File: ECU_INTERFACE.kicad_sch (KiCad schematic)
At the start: 14 parts, among them J10 5569-16A2, J2 5569-20A2, J3 5569-06A2, J4 5569-08A2, J5 5569-18A2

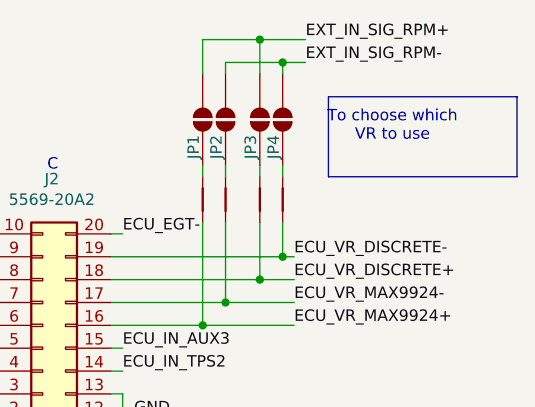
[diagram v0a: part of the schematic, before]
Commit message: Autosave
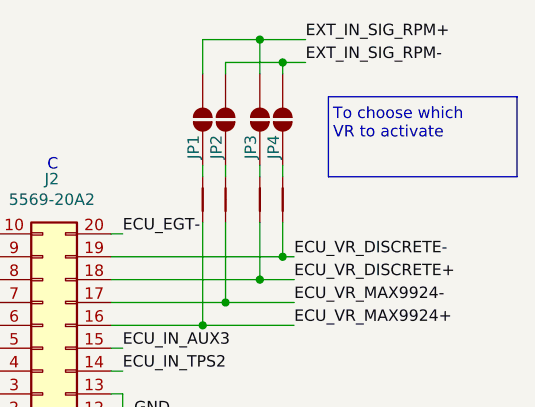
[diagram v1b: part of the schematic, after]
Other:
- note added: "To choose which VR to activate"
- note removed: "To choose which VR to use"
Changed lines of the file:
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@@
 		)
 	)
-	(text "To choose which\nVR to use"
+	(text "To choose which\nVR to activate"
 		(exclude_from_sim no)
-		(at 233.172 52.832 0)
+		(at 226.568 52.578 0)
 		(effects
 			(font
 				(size 1.27 1.27)
 			)
+			(justify left)
 		)
 	)
